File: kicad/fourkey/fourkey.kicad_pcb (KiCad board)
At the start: 2 copper layers, 40 x 64 mm, 5 parts, among them U1 TEENSY2.0

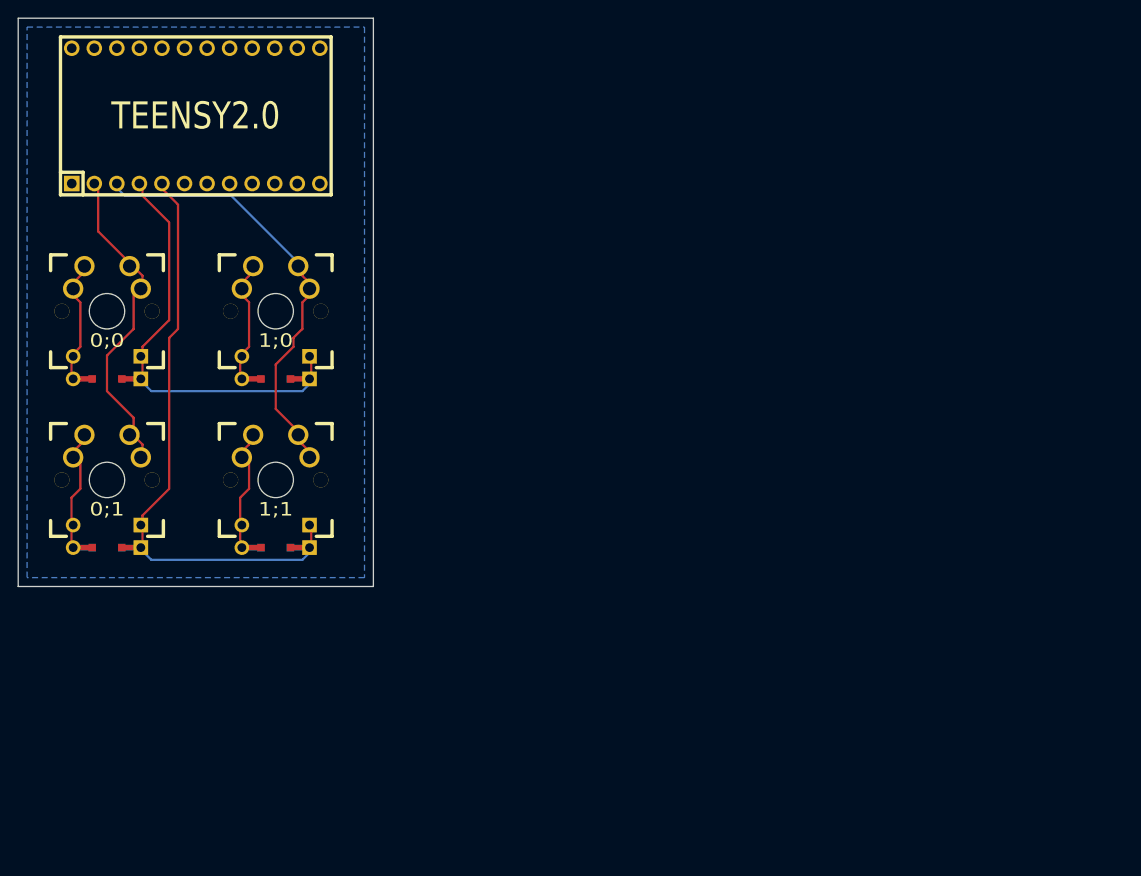
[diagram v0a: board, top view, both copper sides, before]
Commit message: Mostly fourkey PCB work
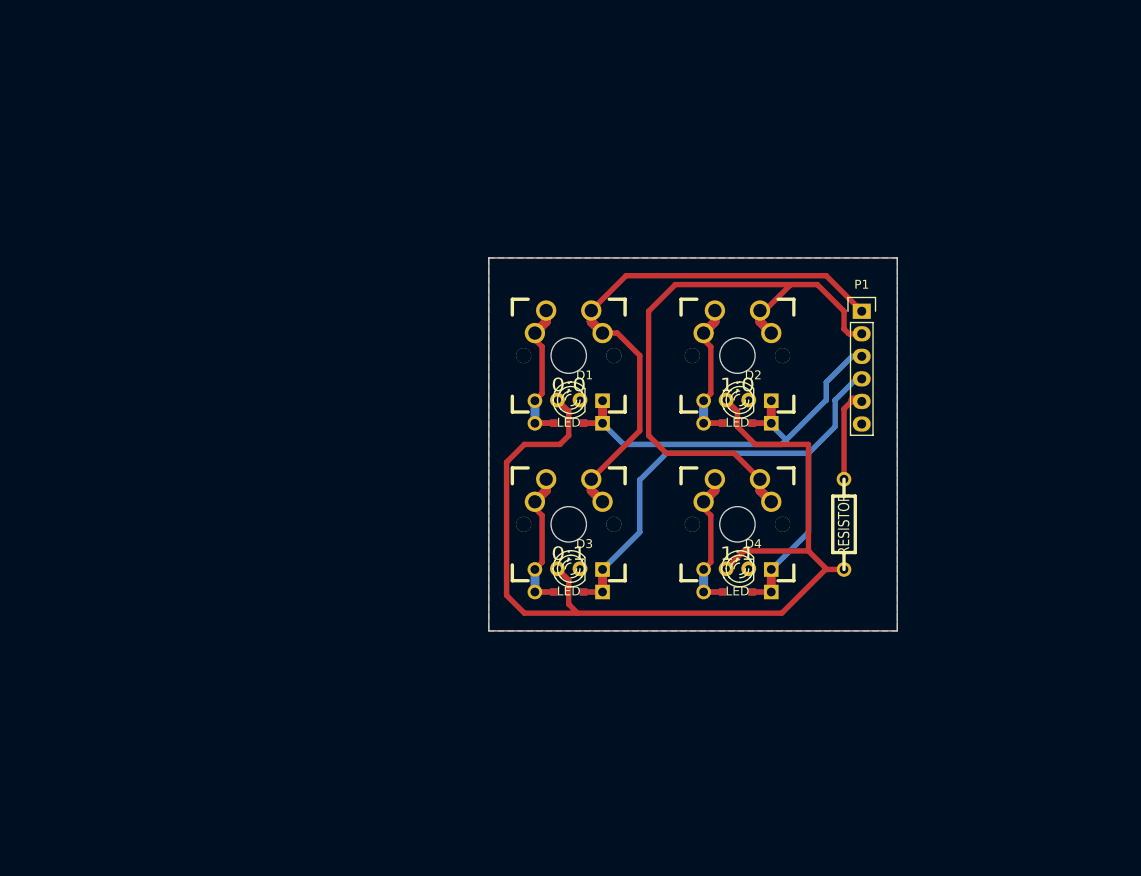
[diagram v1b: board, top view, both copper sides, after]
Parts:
- removed U1: TEENSY2.0, footprint:TEENSY_2.0
- added D1: LED, LEDs:LED-3MM, F.Cu at (154.0, 113.0)
- added D2: LED, LEDs:LED-3MM, F.Cu at (173.0, 113.0)
- added D3: LED, LEDs:LED-3MM, F.Cu at (154.0, 132.0)
- added D4: LED, LEDs:LED-3MM, F.Cu at (173.0, 132.0)
- added P1: CONN_01X06, Pin_Headers:Pin_Header_Straight_1x06, F.Cu at (187.0, 103.0)
- added R1: RESISTOR, footprint:RESISTOR, F.Cu at (185.0, 127.0)
- moved 0;0 52.2 mm to (154.0, 108.0)
- moved 0;1 52.2 mm to (154.0, 127.0)
- moved 1;0 52.2 mm to (173.0, 108.0)
- moved 1;1 52.2 mm to (173.0, 127.0)
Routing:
- net Net-(D1-Pad1): track 0.00 -> 112.0 mm
- net /COL0: track 39.3 -> 67.4 mm
- net /COL1: track 53.2 -> 74.2 mm
- net /LED: track 0.00 -> 10.5 mm
- net /ROW0: track 50.1 -> 43.1 mm
- net /ROW1: track 69.1 -> 63.2 mm
- added copper zone on F.Cu, net GND
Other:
- board size 40 x 64 mm -> 46 x 42 mm

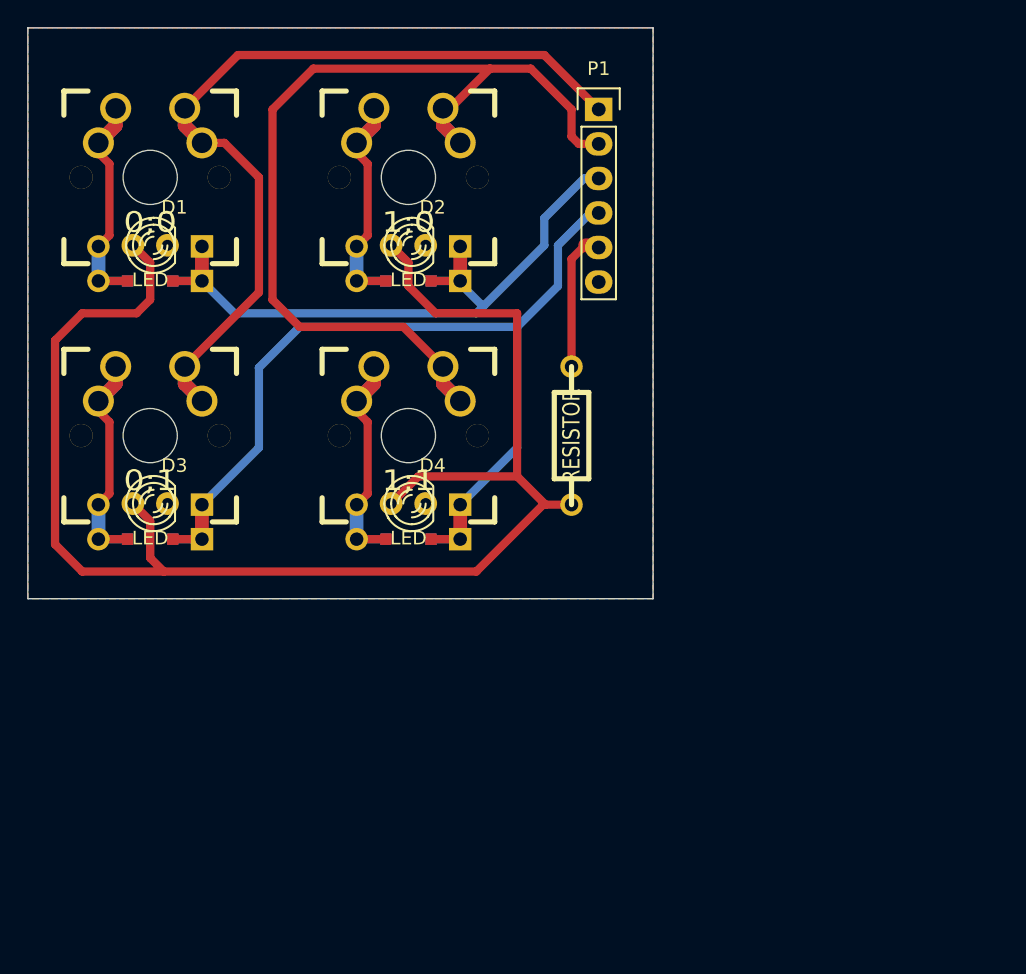
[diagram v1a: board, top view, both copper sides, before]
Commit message: More FourKey work, including Gerber files
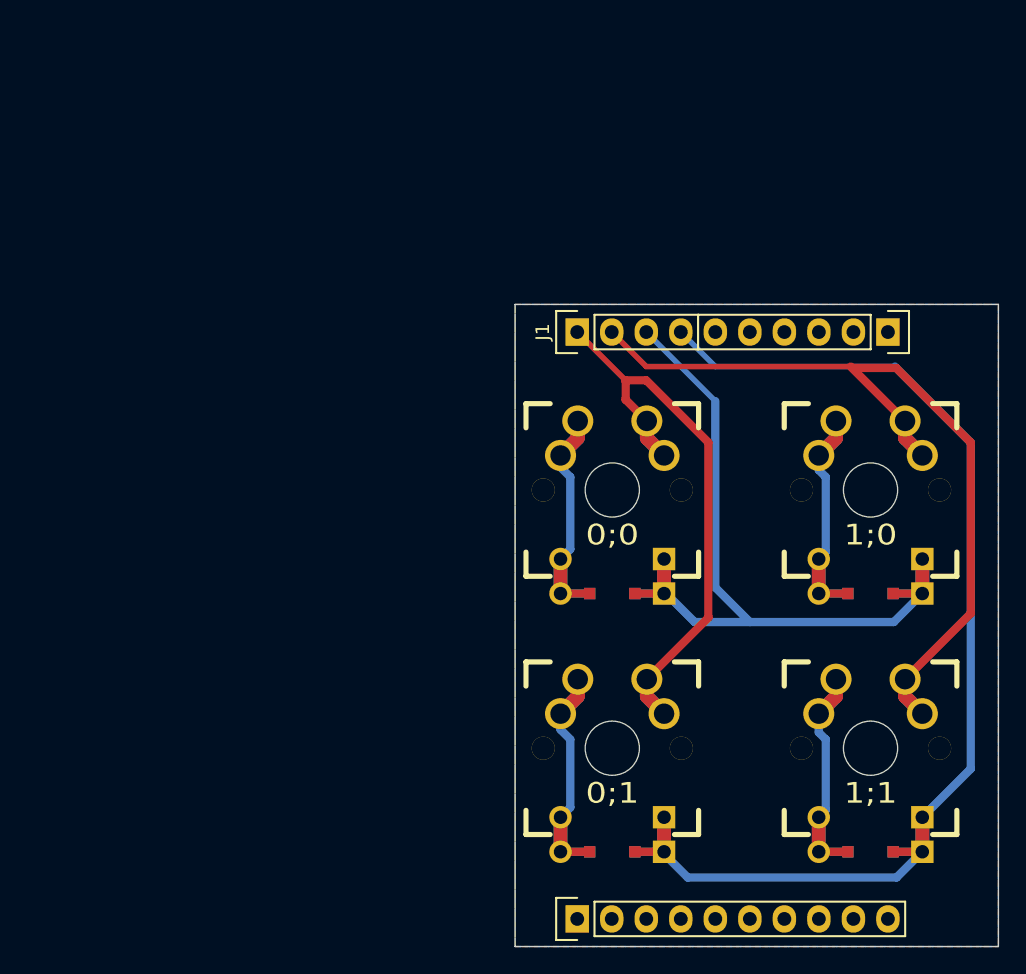
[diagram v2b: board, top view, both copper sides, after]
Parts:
- removed D1, D2, D3, D4: LED, LEDs:LED-3MM
- removed P1: CONN_01X06, Pin_Headers:Pin_Header_Straight_1x06
- removed R1: RESISTOR, footprint:RESISTOR
- added J1: 4PIN, Pin_Headers:Pin_Header_Straight_1x04, F.Cu at (185.4, 119.4)
- added Pin_Header_Straight_1x06: VAL**, Pin_Headers:Pin_Header_Straight_1x06, F.Cu at (208.3, 119.4)
- added Pin_Header_Straight_1x10: VAL**, Pin_Headers:Pin_Header_Straight_1x10, F.Cu at (185.4, 162.6)
- moved 0;0 41.0 mm to (188.0, 131.0)
- moved 0;1 41.0 mm to (188.0, 150.0)
- moved 1;0 41.0 mm to (207.0, 131.0)
- moved 1;1 41.0 mm to (207.0, 150.0)
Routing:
- net Net-(D1-Pad1): track 112.0 -> 0.00 mm
- net /ROW1: track 63.2 -> 84.6 mm
- net /COL0: track 67.4 -> 49.3 mm
- net /ROW0: track 43.1 -> 55.4 mm
- net /LED: track 10.5 -> 0.00 mm
- net /COL1: track 74.2 -> 67.0 mm
- net Net-(0;1-Pad2): track 17.0 -> 19.4 mm
- net Net-(0;0-Pad2): track 17.0 -> 19.4 mm
- net Net-(1;1-Pad2): track 17.0 -> 19.3 mm
- net Net-(1;0-Pad2): track 17.0 -> 19.3 mm
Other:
- board size 46 x 42 mm -> 35.6 x 47.2 mm
